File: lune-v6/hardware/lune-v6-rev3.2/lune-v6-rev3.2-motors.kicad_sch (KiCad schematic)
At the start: 30 parts, among them J11 MOTOR 1 4P4C, J12 MOTOR 2 4P4C, J13 MOTOR 3 4P4C, J14 MOTOR 4 4P4C, J15 MOTOR 5 4P4C, J16 MOTOR 6 4P4C, U20 DRV8411PWPR, U21 DRV8411PWPR, U22 DRV8411PWPR, U40 USBLC6-4SC6 MOTOR ESD, U41 USBLC6-4SC6 MOTOR ESD, U42 USBLC6-4SC6 MOTOR ESD

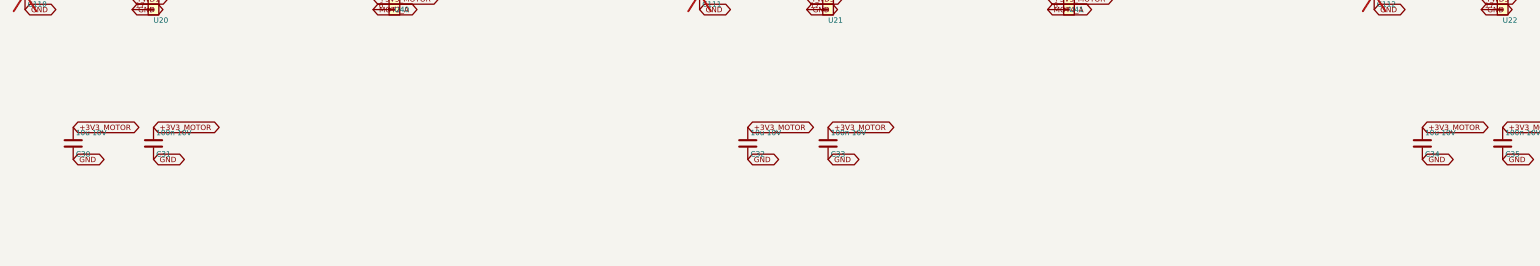
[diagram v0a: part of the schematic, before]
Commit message: Refactor code structure for improved readability and maintainability
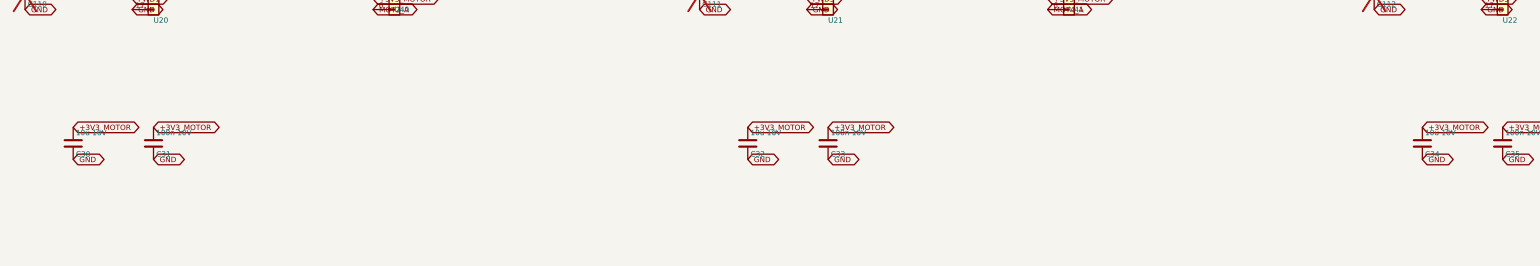
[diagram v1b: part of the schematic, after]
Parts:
- C30, C32, C34: value 10u 10V -> 10u 16V; footprint Capacitor_SMD:C_0805_2012Metric -> Capacitor_SMD:C_0603_1608Metric; Dielectric (none) -> X5R_RATIFIED_VERIFY_EFFECTIVE_C_AT_3V3; LCSC C380346 -> C18164635; MPN TCC0805X7R106K100FT -> TCC0603X5R106K160CT
- RSA1, RSA2, RSA3, RSB1, RSB2, RSB3: footprint Resistor_SMD:R_1206_3216Metric -> Resistor_SMD:R_0603_1608Metric; LCSC C346773 -> C112305; MPN CSR1206FK1R00 -> RC0603FR-071RL

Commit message: Add placement floorplan SVG and geometry JSON for Lune V6 rev3.2
- Introduced a new SVG file for the component placement floorplan, detailing the layout and dimensions of the Lune V6 rev3.2 hardware.
- Added a JSON file containing the geometric coordinates for each component, including reference designators and their respective positions on the board.
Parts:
- removed C110, C111, C112: 2.2u DNP DRV8833, Capacitor_SMD:C_0603_1608Metric, symbol Device:C
- removed C114, C115, C116: 10n DNP DRV8833, Capacitor_SMD:C_0603_1608Metric, symbol Device:C
- removed U40, U41, U42: USBLC6-4SC6 MOTOR ESD, Package_TO_SOT_SMD:SOT-23-6, symbol Connector_Generic:Conn_01x06
- added D40, D41, D42, D43, D44, D45, D46, D47, D48, D49, D50, D51: TPD1E10B06 ESD, Diode_SMD:D_SOD-523, symbol Device:D_TVS
- U20, U21, U22: Pinout 1 nSLEEP; 2 AOUT1; 3 AISEN; 4 AOUT2; 5 BOUT2; 6 BISEN; 7 BOUT1; 8 nFAULT; 9 BIN1; 10 BIN2; 11 NC/VCP fallback; 12 VM; 13 GND; 14 NC/VINT fallback; 15 AIN2; 16 AIN1; 17 EP -> 1 nSLEEP; 2 AOUT1; 3 AISEN; 4 AOUT2; 5 BOUT2; 6 BISEN; 7 BOUT1; 8 nFAULT; 9 BIN1; 10 BIN2; 11 NC (VCP on die); 12 VM; 13 GND; 14 NC (VINT on die); 15 AIN2; 16 AIN1; 17 EP
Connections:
- net GND: now also D40.2 (A2), D41.2 (A2), D42.2 (A2), D43.2 (A2), D44.2 (A2), D45.2 (A2), D46.2 (A2), D47.2 (A2), D48.2 (A2), D49.2 (A2), D50.2 (A2), D51.2 (A2)
- net MOT1_A: now also D40.1 (A1)
- net MOT1_B: now also D41.1 (A1)
- net MOT2_A: now also D42.1 (A1)
- net MOT2_B: now also D43.1 (A1)
- net MOT3_A: now also D44.1 (A1)
- net MOT3_B: now also D45.1 (A1)
- net MOT4_A: now also D46.1 (A1)
- net MOT4_B: now also D47.1 (A1)
- net MOT5_A: now also D48.1 (A1)
- net MOT5_B: now also D49.1 (A1)
- net MOT6_A: now also D50.1 (A1)
- net MOT6_B: now also D51.1 (A1)
- net VCP1: no longer names the net of U20.11 (Pin_11)
- net VCP2: no longer names the net of U21.11 (Pin_11)
- net VCP3: no longer names the net of U22.11 (Pin_11)
- net VINT1: no longer names the net of U20.14 (Pin_14)
- net VINT2: no longer names the net of U21.14 (Pin_14)
- net VINT3: no longer names the net of U22.14 (Pin_14)
- no-connect marks 12 -> 18
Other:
- note added: "Motor ESD is one GND-referenced TPD1E10B06 per wire at its own connector pin. Do not substitute a rail-clamp"
- note added: "array (USBLC6 class): its VBUS pin steers positive strikes into +3V3_MOTOR, i.e. into DRV8411 VM and INA180 IN-."
